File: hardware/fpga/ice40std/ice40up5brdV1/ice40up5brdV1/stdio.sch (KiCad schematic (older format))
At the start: 11 parts, among them J1 Conn_01x20_Male, J2 Conn_01x20_Female

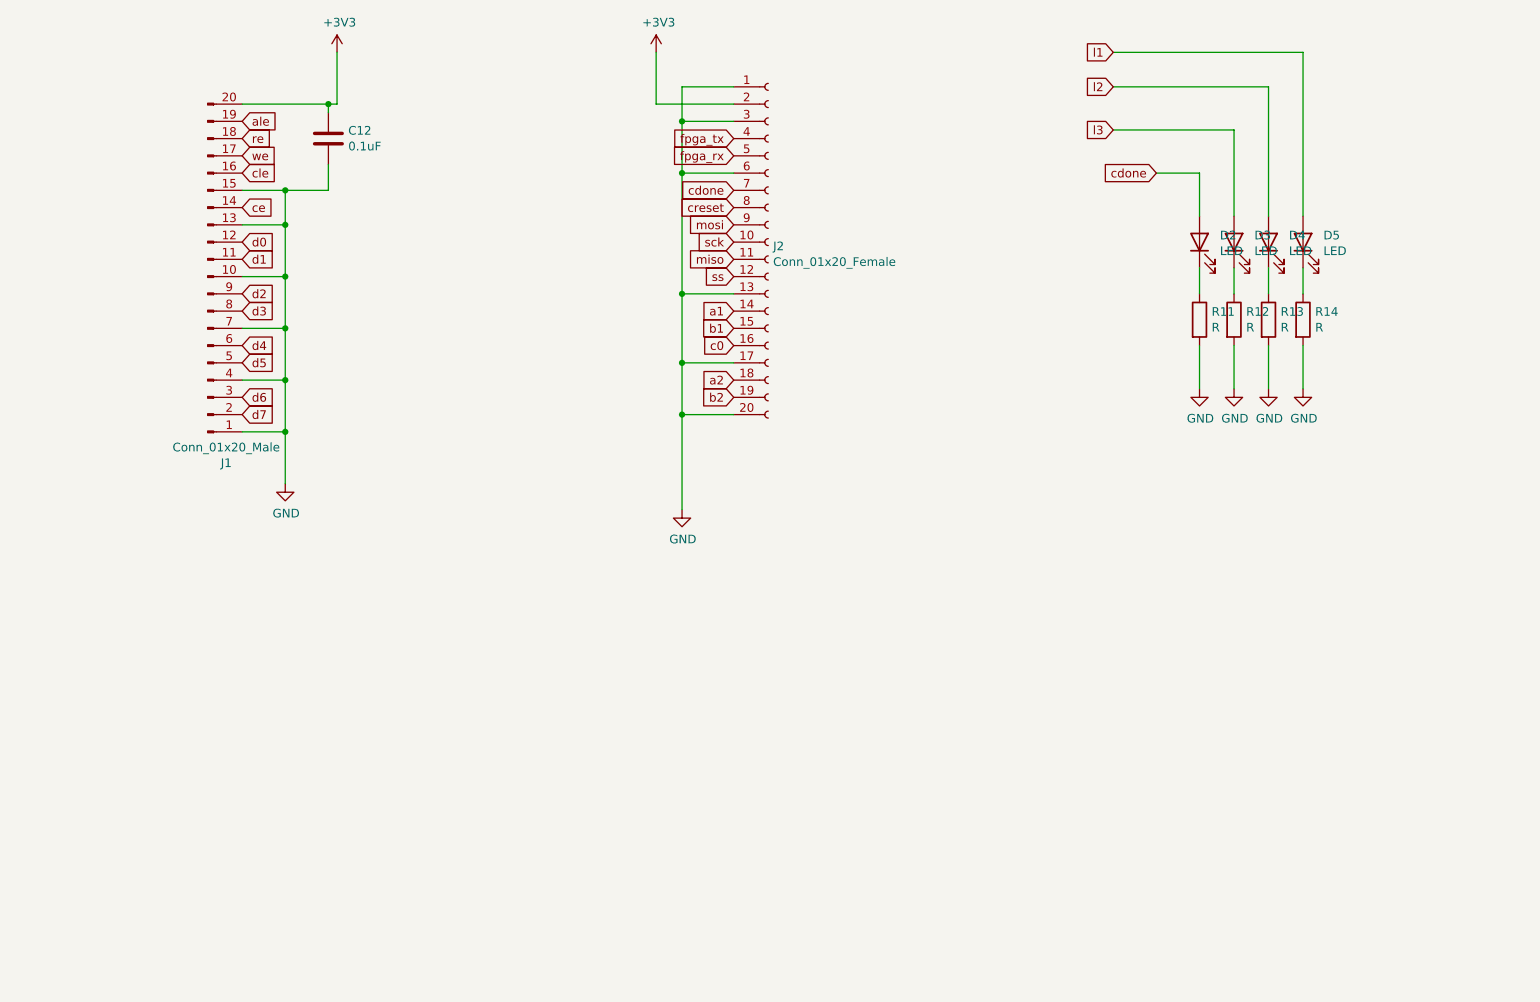
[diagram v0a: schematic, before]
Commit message: FPGA improvements, SPEC changed!
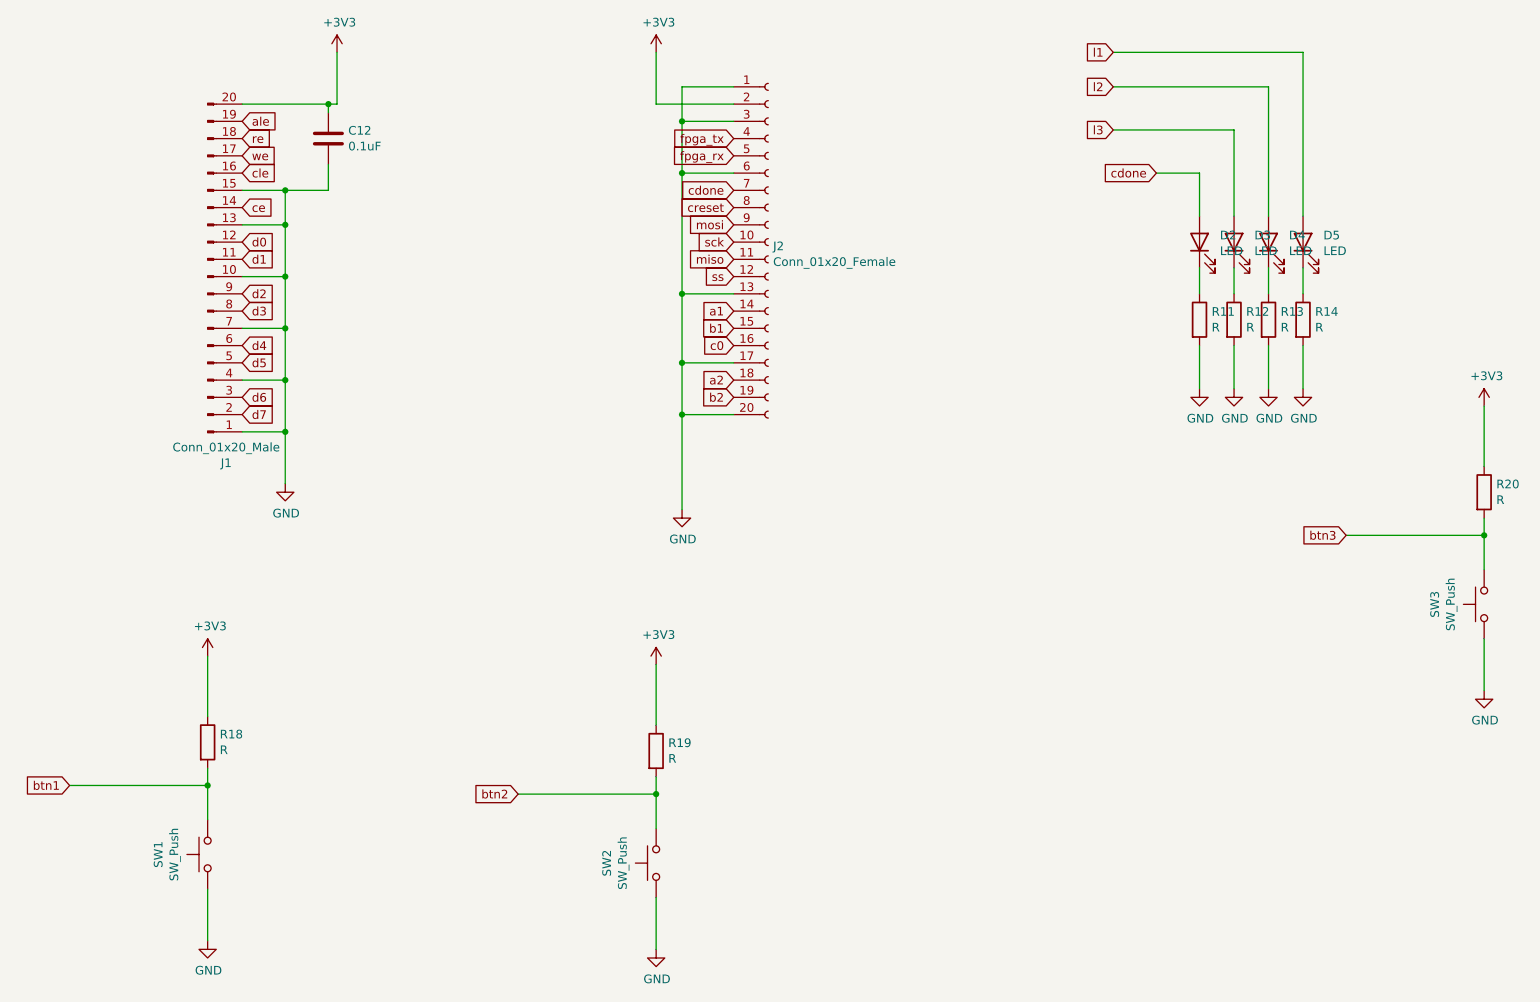
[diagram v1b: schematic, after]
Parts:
- added R18, R19, R20: R, Resistor_SMD:R_0402_1005Metric, symbol Device:R
- added SW1, SW2, SW3: SW_Push, Button_Switch_THT:SW_PUSH_6mm_H8mm, symbol Switch:SW_Push
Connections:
- net +3V3: now also R18.1, R19.1, R20.1
- net GND: now also SW1.1, SW2.1, SW3.1
- new net btn1: R18.2, SW1.2
- new net btn2: R19.2, SW2.2
- new net btn3: R20.2, SW3.2
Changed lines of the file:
@@
 Wire Wire Line
 	5200 2550 5200 3250
+$Comp
+L Switch:SW_Push SW3
+U 1 1 60B5A3BF
+P 9850 5050
+F 0 "SW3" H 9850 5335 50  0000 C CNN
+F 1 "SW_Push" H 9850 5244 50  0000 C CNN
+F 2 "Button_Switch_THT:SW_PUSH_6mm_H8mm" H 9850 5250 50  0001 C CNN
+F 3 "~" H 9850 5250 50  0001 C CNN
+	1    9850 5050
+	0    -1   -1   0
+$EndComp
+$Comp
+L Device:R R20
+U 1 1 60B5E8C2
+P 9850 4400
+F 0 "R20" H 9920 4446 50  0000 L CNN
+F 1 "R" H 9920 4355 50  0000 L CNN
+F 2 "Resistor_SMD:R_0402_1005Metric" V 9780 4400 50  0001 C CNN
+F 3 "~" H 9850 4400 50  0001 C CNN
+	1    9850 4400
+	1    0    0    -1
+$EndComp
+$Comp
+L power:+3V3 #PWR058
+U 1 1 60B66E1C
+P 9850 3900
+F 0 "#PWR058" H 9850 3750 50  0001 C CNN
+F 1 "+3V3" H 9865 4073 50  0000 C CNN
+F 2 "" H 9850 3900 50  0001 C CNN
+F 3 "" H 9850 3900 50  0001 C CNN
+	1    9850 3900
+	1    0    0    -1
+$EndComp
+Wire Wire Line
+	9850 3900 9850 4250
+Wire Wire Line
+	9850 4550 9850 4650
+$Comp
+L power:GND #PWR059
+U 1 1 60B6A246
+P 9850 5550
+F 0 "#PWR059" H 9850 5300 50  0001 C CNN
+F 1 "GND" H 9855 5377 50  0000 C CNN
+F 2 "" H 9850 5550 50  0001 C CNN
+F 3 "" H 9850 5550 50  0001 C CNN
+	1    9850 5550
+	1    0    0    -1
+$EndComp
+Wire Wire Line
+	9850 5250 9850 5550
+Text GLabel 9050 4650 0    50   Input ~ 0
+btn3
+Wire Wire Line
+	9050 4650 9850 4650
+Connection ~ 9850 4650
+Wire Wire Line
+	9850 4650 9850 4850
+$Comp
+L Switch:SW_Push SW1
+U 1 1 60B72AC5
+P 2450 6500
+F 0 "SW1" H 2450 6785 50  0000 C CNN
+F 1 "SW_Push" H 2450 6694 50  0000 C CNN
+F 2 "Button_Switch_THT:SW_PUSH_6mm_H8mm" H 2450 6700 50  0001 C CNN
+F 3 "~" H 2450 6700 50  0001 C CNN
+	1    2450 6500
+	0    -1   -1   0
+$EndComp
+$Comp
+L Device:R R18
+U 1 1 60B72ACB
+P 2450 5850
+F 0 "R18" H 2520 5896 50  0000 L CNN
+F 1 "R" H 2520 5805 50  0000 L CNN
+F 2 "Resistor_SMD:R_0402_1005Metric" V 2380 5850 50  0001 C CNN
+F 3 "~" H 2450 5850 50  0001 C CNN
+	1    2450 5850
+	1    0    0    -1
+$EndComp
+$Comp
+L power:+3V3 #PWR022
+U 1 1 60B72AD1
+P 2450 5350
+F 0 "#PWR022" H 2450 5200 50  0001 C CNN
+F 1 "+3V3" H 2465 5523 50  0000 C CNN
+F 2 "" H 2450 5350 50  0001 C CNN
+F 3 "" H 2450 5350 50  0001 C CNN
+	1    2450 5350
+	1    0    0    -1
+$EndComp
+Wire Wire Line
+	2450 5350 2450 5700
+Wire Wire Line
+	2450 6000 2450 6100
+$Comp
+L power:GND #PWR046
+U 1 1 60B72AD9
+P 2450 7000
+F 0 "#PWR046" H 2450 6750 50  0001 C CNN
+F 1 "GND" H 2455 6827 50  0000 C CNN
+F 2 "" H 2450 7000 50  0001 C CNN
+F 3 "" H 2450 7000 50  0001 C CNN
+	1    2450 7000
+	1    0    0    -1
+$EndComp
+Wire Wire Line
+	2450 6700 2450 7000
+Text GLabel 1650 6100 0    50   Input ~ 0
+btn1
+Wire Wire Line
+	1650 6100 2450 6100
+Connection ~ 2450 6100
+Wire Wire Line
+	2450 6100 2450 6300
+$Comp
+L Switch:SW_Push SW2
+U 1 1 60B7479D
+P 5050 6550
+F 0 "SW2" H 5050 6835 50  0000 C CNN
+F 1 "SW_Push" H 5050 6744 50  0000 C CNN
+F 2 "Button_Switch_THT:SW_PUSH_6mm_H8mm" H 5050 6750 50  0001 C CNN
+F 3 "~" H 5050 6750 50  0001 C CNN
+	1    5050 6550
+	0    -1   -1   0
+$EndComp
+$Comp
+L Device:R R19
+U 1 1 60B747A3
+P 5050 5900
+F 0 "R19" H 5120 5946 50  0000 L CNN
+F 1 "R" H 5120 5855 50  0000 L CNN
+F 2 "Resistor_SMD:R_0402_1005Metric" V 4980 5900 50  0001 C CNN
+F 3 "~" H 5050 5900 50  0001 C CNN
+	1    5050 5900
+	1    0    0    -1
+$EndComp
+$Comp
+L power:+3V3 #PWR052
+U 1 1 60B747A9
+P 5050 5400
+F 0 "#PWR052" H 5050 5250 50  0001 C CNN
+F 1 "+3V3" H 5065 5573 50  0000 C CNN
+F 2 "" H 5050 5400 50  0001 C CNN
+F 3 "" H 5050 5400 50  0001 C CNN
+	1    5050 5400
+	1    0    0    -1
+$EndComp
+Wire Wire Line
+	5050 5400 5050 5750
+Wire Wire Line
+	5050 6050 5050 6150
+$Comp
+L power:GND #PWR053
+U 1 1 60B747B1
+P 5050 7050
+F 0 "#PWR053" H 5050 6800 50  0001 C CNN
+F 1 "GND" H 5055 6877 50  0000 C CNN
+F 2 "" H 5050 7050 50  0001 C CNN
+F 3 "" H 5050 7050 50  0001 C CNN
+	1    5050 7050
+	1    0    0    -1
+$EndComp
+Wire Wire Line
+	5050 6750 5050 7050
+Text GLabel 4250 6150 0    50   Input ~ 0
+btn2
+Wire Wire Line
+	4250 6150 5050 6150
+Connection ~ 5050 6150
+Wire Wire Line
+	5050 6150 5050 6350
 $EndSCHEMATC

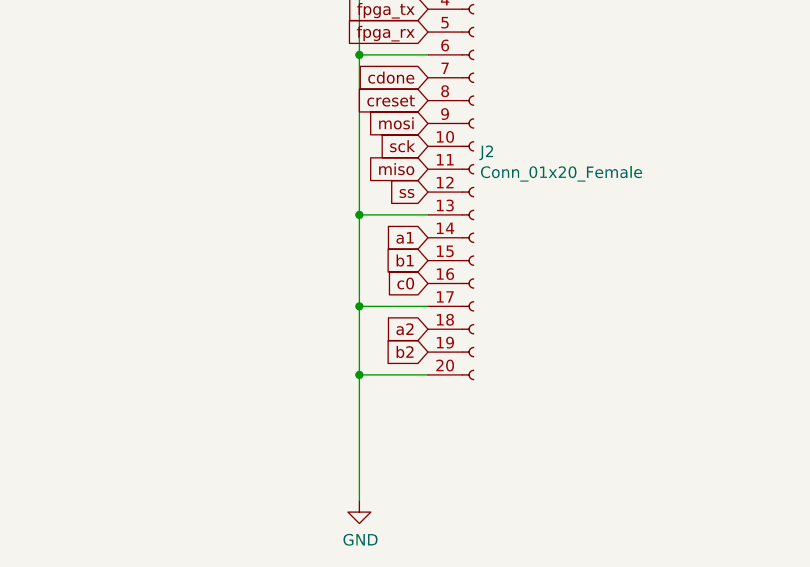
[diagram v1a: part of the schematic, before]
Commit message: FPGA improvements, SPEC changed!
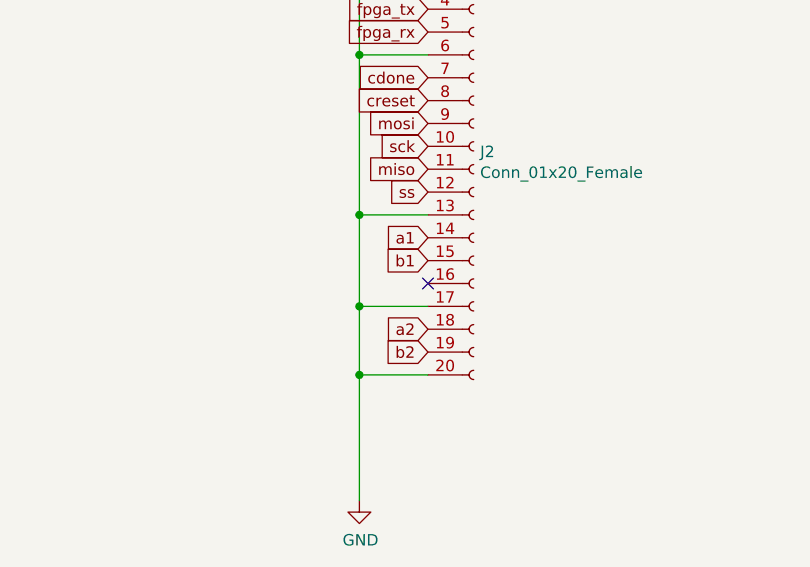
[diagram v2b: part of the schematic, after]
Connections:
- net c0: no longer names the net of J2.16 (Pin_16)
- no-connect marks 0 -> 1
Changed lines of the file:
@@
 Text GLabel 5500 3850 0    50   Input ~ 0
 b2
-Text GLabel 5500 3550 0    50   Input ~ 0
-c0
 Text GLabel 7950 2550 0    50   Input ~ 0
 cdone
@@
 Wire Wire Line
 	5050 6150 5050 6350
+NoConn ~ 5500 3550
 $EndSCHEMATC

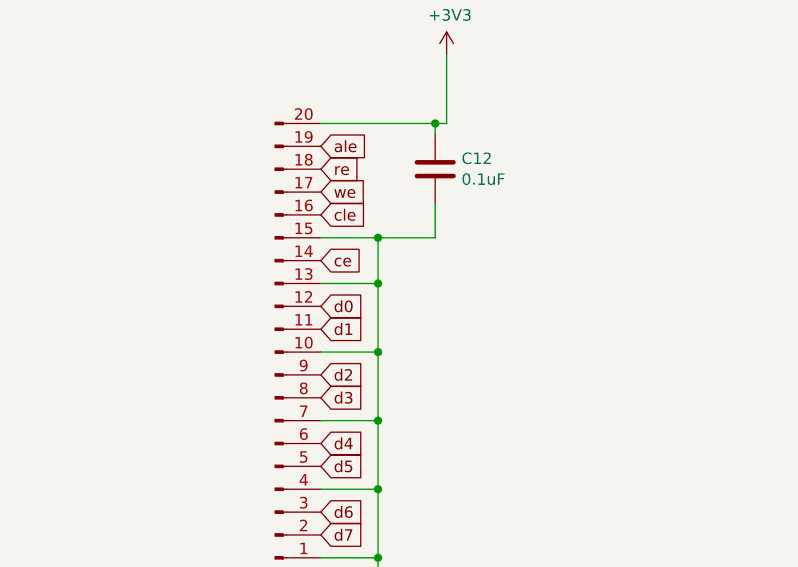
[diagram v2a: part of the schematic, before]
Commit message: ice40qfn restarted: simplest design ready?
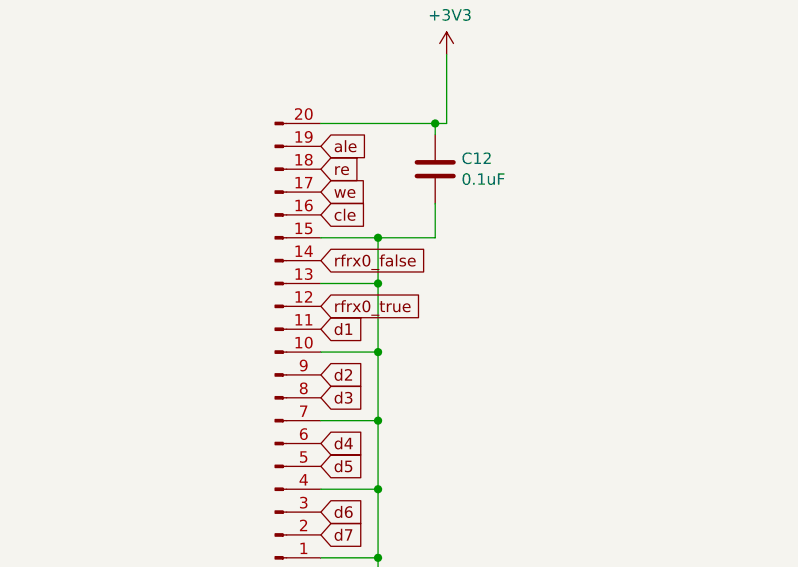
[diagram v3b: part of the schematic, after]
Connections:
- net ce renamed rfrx0_false
- net d0 renamed rfrx0_true
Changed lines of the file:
@@
 cle
 Text GLabel 2650 2750 2    50   Input ~ 0
-ce
+rfrx0_false
 Text GLabel 2650 2950 2    50   Input ~ 0
-d0
+rfrx0_true
 Text GLabel 2650 3050 2    50   Input ~ 0
 d1

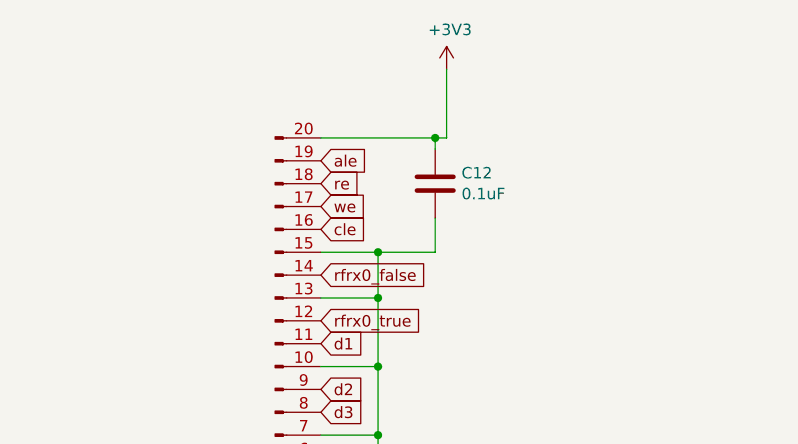
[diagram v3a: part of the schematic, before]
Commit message: ice40qfn restarted: simplest design ready?
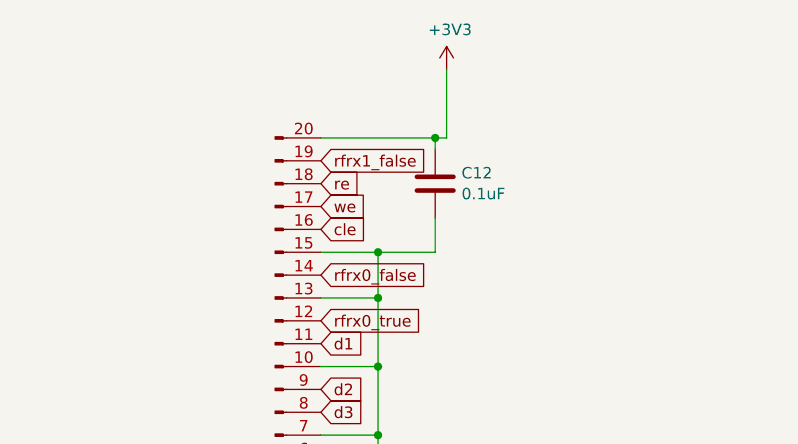
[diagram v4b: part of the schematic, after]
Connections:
- net ale renamed rfrx1_false
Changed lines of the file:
@@
 	8800 1850 8800 2800
 Text GLabel 2650 2250 2    50   Input ~ 0
-ale
+rfrx1_false
 Text GLabel 2650 2350 2    50   Input ~ 0
 re

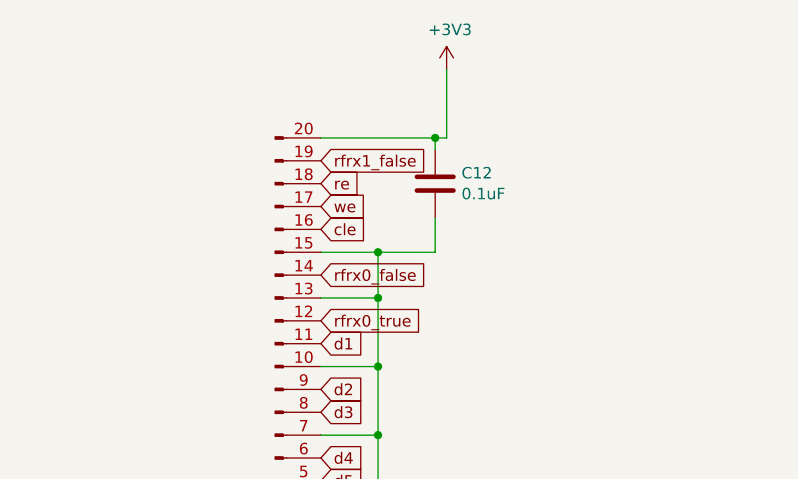
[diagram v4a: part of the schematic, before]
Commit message: ice40qfn restarted: simplest design ready?
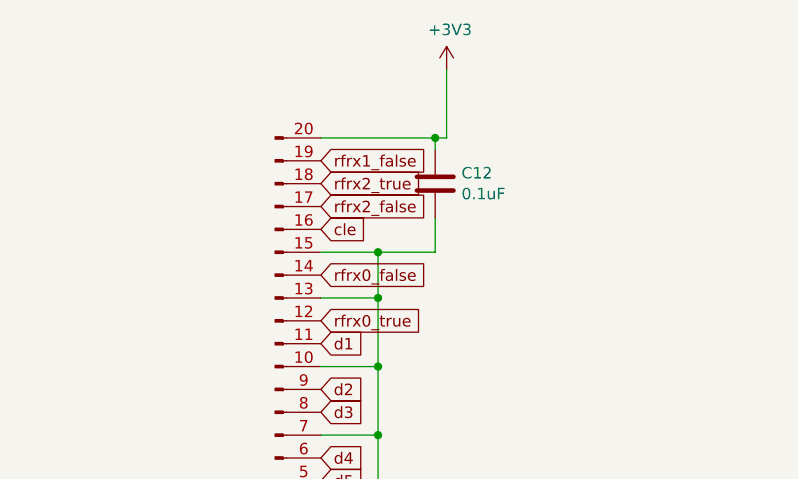
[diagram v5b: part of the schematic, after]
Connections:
- net re renamed rfrx2_true
- net we renamed rfrx2_false
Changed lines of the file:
@@
 rfrx1_false
 Text GLabel 2650 2350 2    50   Input ~ 0
-re
+rfrx2_true
 Text GLabel 2650 2450 2    50   Input ~ 0
-we
+rfrx2_false
 Text GLabel 2650 2550 2    50   Input ~ 0
 cle

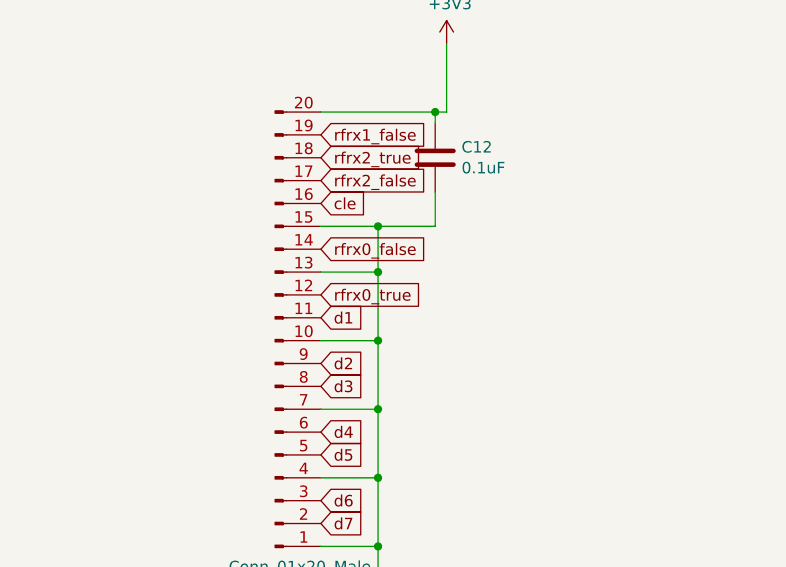
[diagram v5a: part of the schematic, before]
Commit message: ice40qfn restarted: simplest design ready?
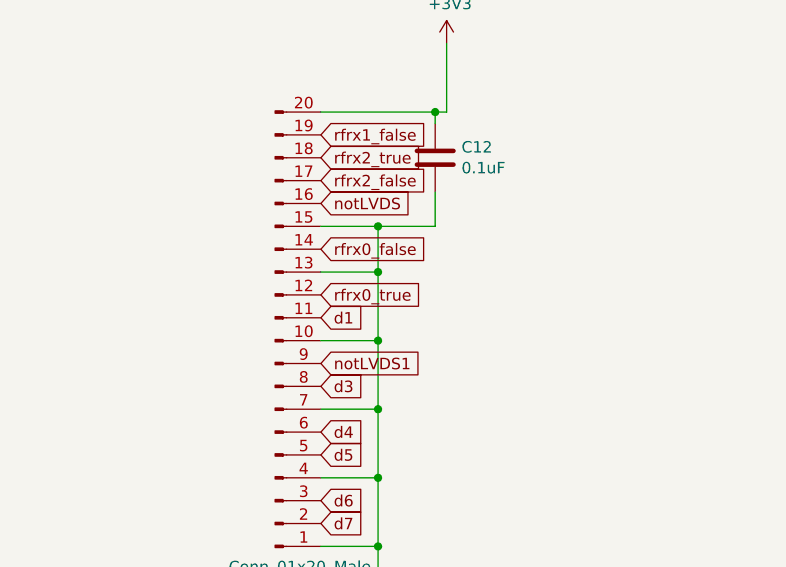
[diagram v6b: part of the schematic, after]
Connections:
- net cle renamed notLVDS
- net d2 renamed notLVDS1
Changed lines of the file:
@@
 rfrx2_false
 Text GLabel 2650 2550 2    50   Input ~ 0
-cle
+notLVDS
 Text GLabel 2650 2750 2    50   Input ~ 0
 rfrx0_false
@@
 d1
 Text GLabel 2650 3250 2    50   Input ~ 0
-d2
+notLVDS1
 Text GLabel 2650 3350 2    50   Input ~ 0
 d3
